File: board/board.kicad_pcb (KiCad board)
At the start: 2 copper layers, 21 x 13 mm, 1 part

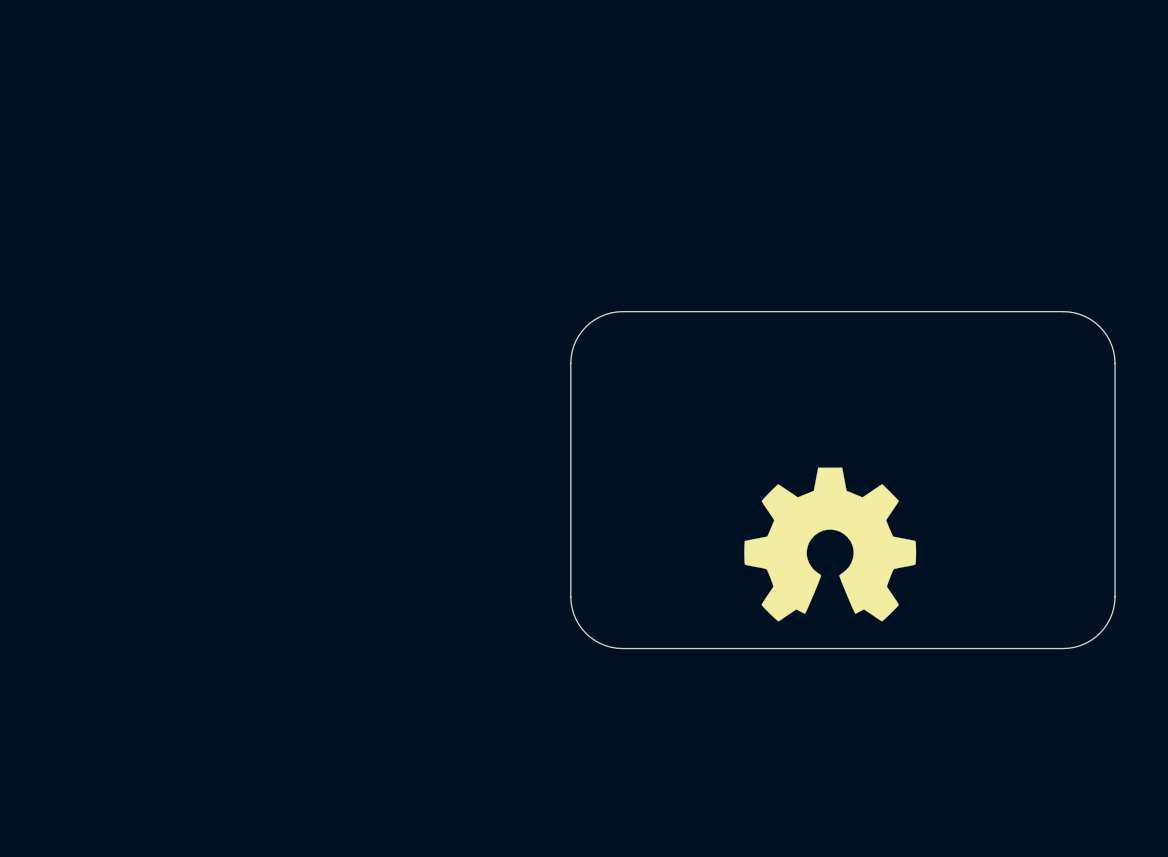
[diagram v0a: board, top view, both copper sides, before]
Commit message: imported legacy version
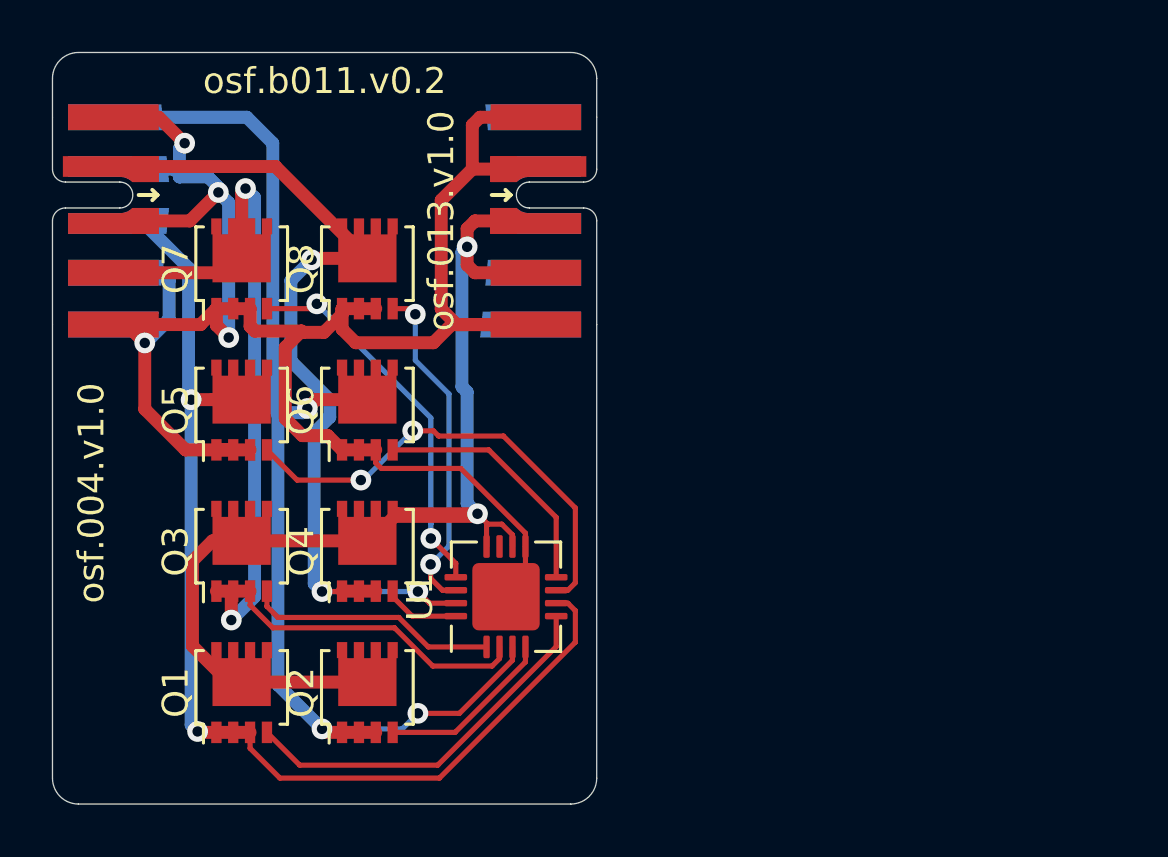
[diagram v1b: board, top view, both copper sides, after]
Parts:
- added J1: 004_BASE-T_CT_2x3, on_edge:on_edge_2x05_device, F.Cu at (120.0, 86.5)
- added J2: 013_PoE_rectified, on_edge:on_edge_2x05_host, F.Cu at (141.0, 86.5)
- added Q1: TPN3300ANH,LQ, Package_TO_SOT_SMD:LFPAK33, F.Cu at (127.3, 104.7)
- added Q2: TPN3300ANH,LQ, Package_TO_SOT_SMD:LFPAK33, F.Cu at (132.2, 104.7)
- added Q3: TPN3300ANH,LQ, Package_TO_SOT_SMD:LFPAK33, F.Cu at (127.3, 99.2)
- added Q4: TPN3300ANH,LQ, Package_TO_SOT_SMD:LFPAK33, F.Cu at (132.2, 99.2)
- added Q5: TPN3300ANH,LQ, Package_TO_SOT_SMD:LFPAK33, F.Cu at (127.3, 93.8)
- added Q6: TPN3300ANH,LQ, Package_TO_SOT_SMD:LFPAK33, F.Cu at (132.2, 93.8)
- added Q7: TPN3300ANH,LQ, Package_TO_SOT_SMD:LFPAK33, F.Cu at (127.3, 88.3)
- added Q8: TPN3300ANH,LQ, Package_TO_SOT_SMD:LFPAK33, F.Cu at (132.2, 88.3)
- added U1: LT4321, Package_DFN_QFN:WQFN-16-1EP_4x4mm_P0.5mm_EP2.6x2.6mm, F.Cu at (137.5, 101.0)
- LOGO1: footprint Symbol:OSHW-Symbol_6.7x6mm_SilkScreen -> Symbol:OSHW-Logo2_9.8x8mm_SilkScreen; moved to B.Cu
- moved LOGO1 25.1 mm to (125.5, 104.5), turned to 180 degrees
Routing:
- net GND: track 0.00 -> 90.0 mm, vias 0 -> 4
- net /snippet/VPORTP: track 0.00 -> 46.2 mm, vias 0 -> 2
- net /snippet/CT_78: track 0.00 -> 44.9 mm, vias 0 -> 2
- net /snippet/CT_45: track 0.00 -> 44.7 mm, vias 0 -> 3
- net /snippet/CT_36: track 0.00 -> 42.9 mm, vias 0 -> 2
- net /snippet/CT_12: track 0.00 -> 33.8 mm, vias 0 -> 3
- net /snippet/BG_78: track 0.00 -> 18.1 mm, vias 0 -> 2
- net /snippet/BG_36: track 0.00 -> 14.8 mm, vias 0 -> 2
- net /snippet/TG_78: track 0.00 -> 14.8 mm
- net /snippet/BG_12: track 0.00 -> 13.1 mm, vias 0 -> 2
- net /snippet/TG_36: track 0.00 -> 9.71 mm
- net /snippet/BG_45: track 0.00 -> 9.70 mm
- net /snippet/TG_45: track 0.00 -> 6.83 mm
- net /snippet/TG_12: track 0.00 -> 2.96 mm
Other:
- board size 21 x 13 mm -> 21 x 29 mm
- rule pad_to_mask_clearance: 0 -> 0.051
- board text added: "osf.004.v1.0"
- board text added: "osf.013.v1.0"
- board text added: "osf.b011.v0.2"
